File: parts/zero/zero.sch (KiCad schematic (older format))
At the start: 13 parts, among them J1 Conn_02x02_Odd_Even, J2 Conn_02x04_Odd_Even, J3 Conn_01x02, K1 HK19F

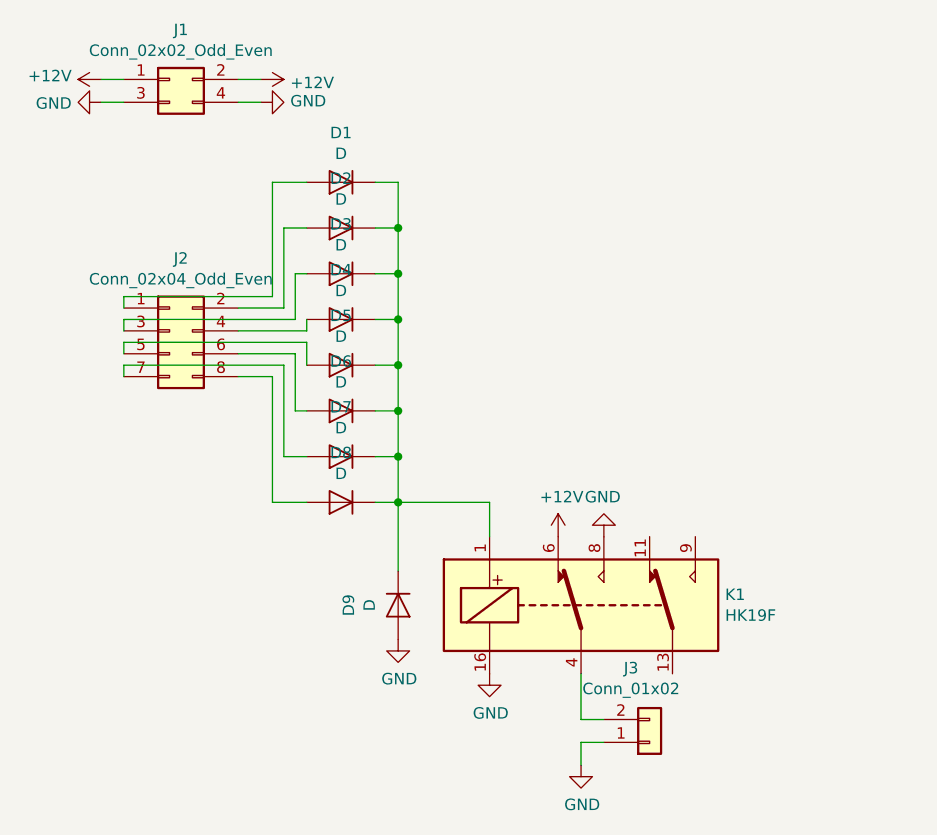
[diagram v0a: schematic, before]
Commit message: Many things happened at 35C3.
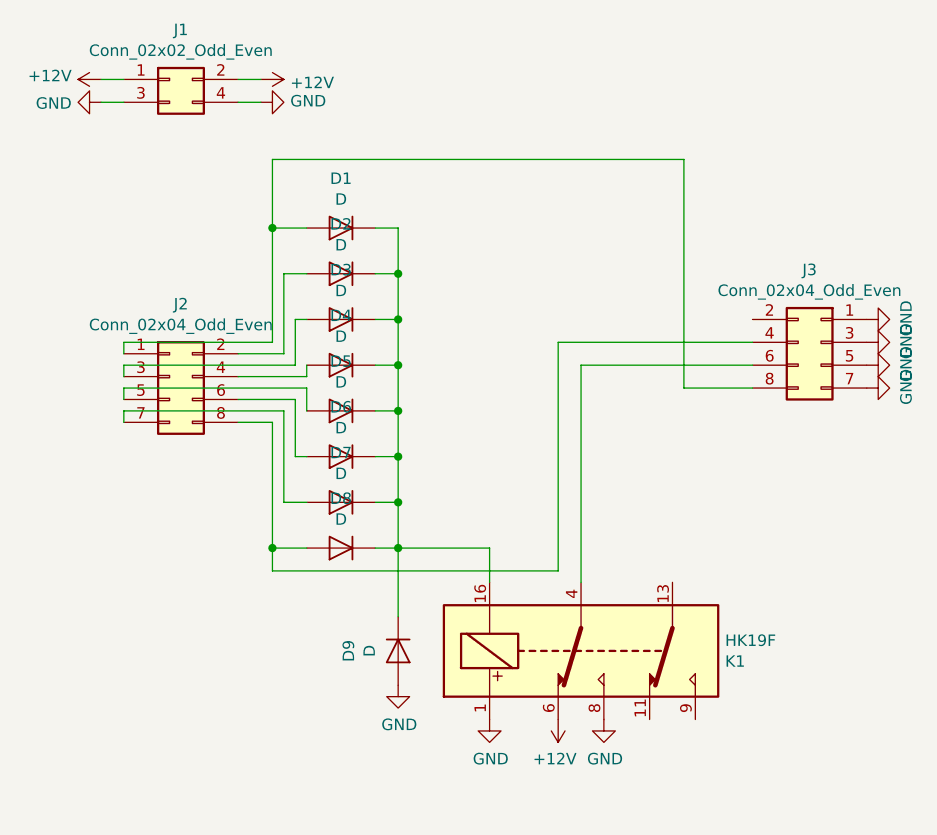
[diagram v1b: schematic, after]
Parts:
- removed J3: Conn_01x02, Pin_Headers:Pin_Header_Straight_1x02_Pitch2.54mm, symbol Connector_Generic:Conn_01x02
- added J3: Conn_02x04_Odd_Even, Pin_Headers:Pin_Header_Straight_2x04_Pitch2.54mm, symbol Connector_Generic:Conn_02x04_Odd_Even
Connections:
- net GND: now also K1.1, J3.1 (Pin_1), J3.3 (Pin_3), J3.5 (Pin_5), J3.7 (Pin_7); no longer K1.16
- net at D1.2 (A), J2.1 (Pin_1): now also J3.8 (Pin_8)
- net at D8.2 (A), J2.8 (Pin_8): now also J3.4 (Pin_4)
- net at D1.1 (K), D2.1 (K), D3.1 (K)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: now also K1.16; no longer K1.1
- net at K1.4: now also J3.6 (Pin_6)
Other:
- moved on the sheet: D1, D2, D3, D4, D5, D6, D7, D8, D9, J2, K1
